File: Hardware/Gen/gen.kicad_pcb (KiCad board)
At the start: 2 copper layers, 149.6 x 62.2 mm, 51 parts, among them J1 Screw_Terminal_01x03, J2 XLR4, J3 XLR3, J4 GAMEN, J5 SHORI, J6 MAE, U1 TPS56339DDCT, U3 TPS560430YDBVR

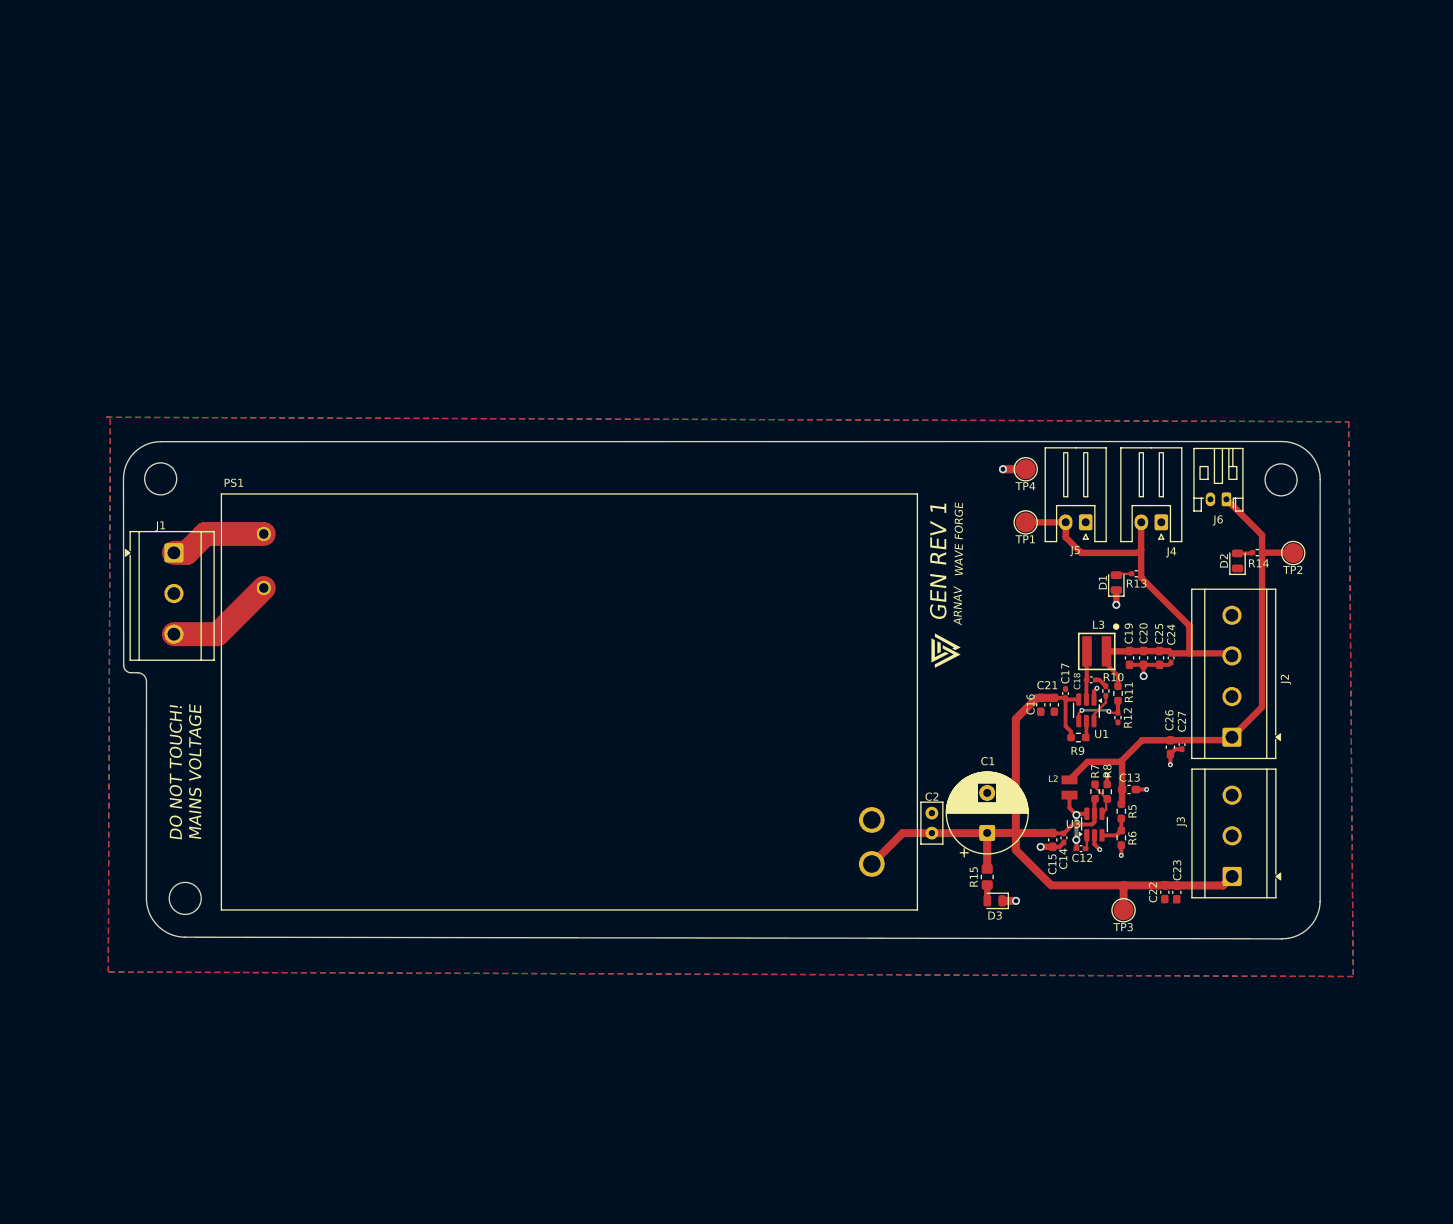
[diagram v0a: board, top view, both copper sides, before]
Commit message: Gen: New Routing, More memes and better buck layouts (rev 2)
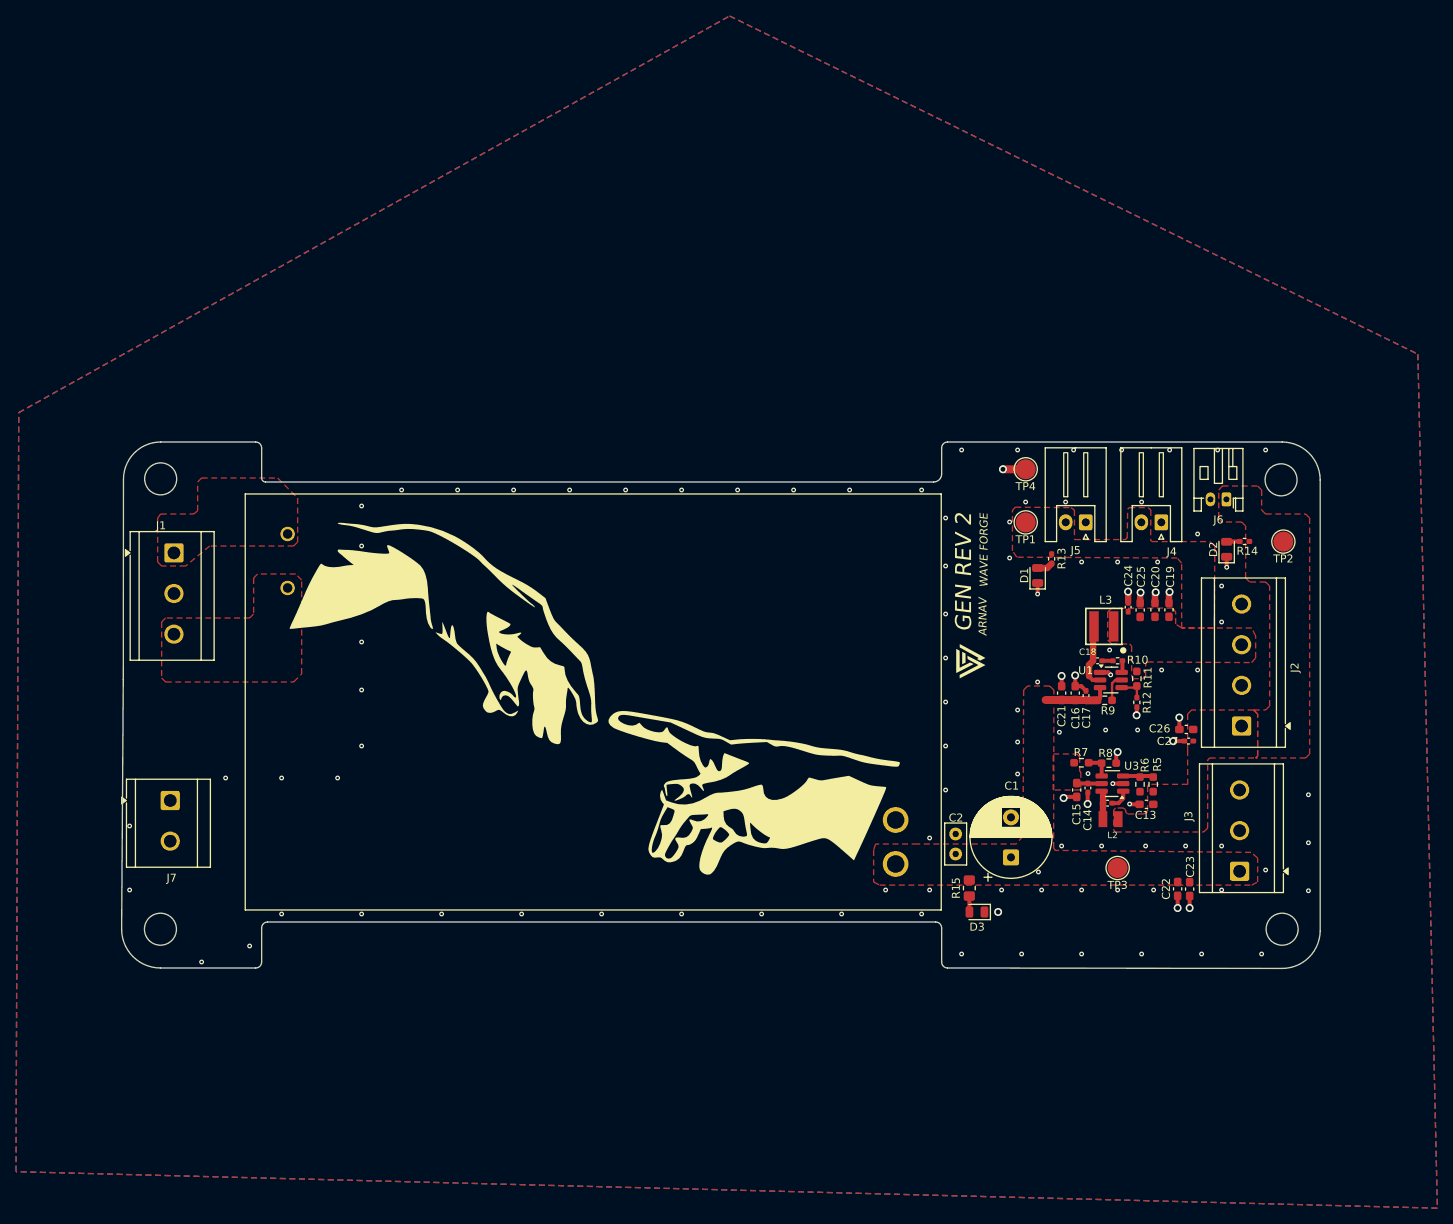
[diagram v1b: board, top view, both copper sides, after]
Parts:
- added G***: LOGO, My footprints:hands, F.Cu at (128.1, 114.7)
- added H3: MountingHole, MountingHole:MountingHole_4mm, F.Cu at (215.1, 141.9)
- added J7: Screw_Terminal_01x02, TerminalBlock_CUI:TerminalBlock_CUI_TB007-508-02_1x02_P5.08mm_Horizontal, F.Cu at (76.1, 125.8)
- moved R13 10.8 mm to (186.2, 95.6), turned to 90 degrees
- moved D1 9.88 mm to (184.5, 97.7)
- moved C24 8.32 mm to (195.8, 101.6), turned to -90 degrees
- moved C19 7.77 mm to (200.9, 102.0), turned to -90 degrees
- moved R6 7.08 mm to (197.3, 123.8)
- moved C14 6.92 mm to (190.8, 124.2)
- moved C15 6.92 mm to (189.4, 124.5)
- moved C12 6.59 mm to (193.2, 126.1)
- moved L2 6.47 mm to (193.6, 128.1), turned to 180 degrees
- moved C25 6.46 mm to (197.3, 102.0), turned to -90 degrees
- moved C20 6.17 mm to (199.2, 102.0), turned to -90 degrees
- moved R9 5.70 mm to (192.9, 113.3)
- moved U3 5.59 mm to (193.8, 123.7), turned to 180 degrees
- moved TP3 5.33 mm to (194.5, 134.2)
- moved R5 5.22 mm to (198.9, 123.8), turned to 90 degrees
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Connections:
- J1 pad 2: GND -> unconnected-(J1-Pin_2-Pad2)
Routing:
- net /DC_OUT: track 101.0 -> 10.9 mm
- net +9V: track 65.0 -> 0.00 mm
- net +5V: track 57.0 -> 0.00 mm
- net /ACL: track 13.6 -> 0.00 mm
- net /ACN: track 12.2 -> 0.00 mm
- net Net-(U3-SW): track 8.65 -> 3.32 mm, vias 2 -> 0
- net Net-(U1-FB): track 7.69 -> 3.44 mm, vias 2 -> 0
- net GND: track 26.6 -> 30.6 mm, vias 11 -> 113
- net Net-(U1-BOOT): track 3.78 -> 1.49 mm
- net Net-(U1-SW): track 6.34 -> 8.07 mm
- net Net-(U1-EN): track 2.09 -> 3.49 mm
- net Net-(U3-EN): track 4.48 -> 3.24 mm
- net Net-(U3-CB): track 1.73 -> 2.53 mm
- added copper zone on F.Cu, net +5V
- added copper zone on F.Cu, net +9V
- added copper zone on F.Cu, net /ACL
- added copper zone on F.Cu, net /ACN
- added copper zone on F.Cu, net /DC_OUT
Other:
- board size 149.6 x 62.2 mm -> 149.8 x 65.8 mm
- board text added: "GEN REV 2"
- board text removed: "DO NOT TOUCH! MAINS VOLTAGE"
- board text removed: "GEN REV 1"
